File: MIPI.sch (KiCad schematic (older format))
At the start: 42 parts, among them J8 49F-1201GYD2NL, J9 MIPI, U1 AllWinner-S3(FBGA-234), Y2 32.768kHz, Y3 24MHz

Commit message: no drc error
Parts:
- R78, R79, R80, R81, R82, R83, R84, R86, R87, R88, R89, R90, R91, R92, R93, R94: footprint otter:C_0402 -> otter:R_0402
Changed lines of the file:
@@
 F 0 "R81" V 2150 1750 50  0000 C CNN
 F 1 "22" V 2150 2050 50  0000 C CNN
-F 2 "otter:C_0402" H 2200 1900 50  0001 C CNN
+F 2 "otter:R_0402" H 2200 1900 50  0001 C CNN
 F 3 "~" H 2200 1900 50  0001 C CNN
 	1    2200 1900
@@
 F 0 "R78" H 1092 3696 50  0000 R CNN
 F 1 "200k" H 1092 3605 50  0000 R CNN
-F 2 "otter:C_0402" H 1150 3650 50  0001 C CNN
+F 2 "otter:R_0402" H 1150 3650 50  0001 C CNN
 F 3 "~" H 1150 3650 50  0001 C CNN
 	1    1150 3650
@@
 F 0 "R87" V 7700 1300 50  0000 C CNN
 F 1 "2k2" V 7700 1650 50  0000 C CNN
-F 2 "otter:C_0402" H 7750 1450 50  0001 C CNN
+F 2 "otter:R_0402" H 7750 1450 50  0001 C CNN
 F 3 "~" H 7750 1450 50  0001 C CNN
 	1    7750 1450
@@
 F 0 "R88" V 7400 1300 50  0000 C CNN
 F 1 "2k2" V 7400 1650 50  0000 C CNN
-F 2 "otter:C_0402" H 7450 1450 50  0001 C CNN
+F 2 "otter:R_0402" H 7450 1450 50  0001 C CNN
 F 3 "~" H 7450 1450 50  0001 C CNN
 	1    7450 1450
@@
 F 0 "R89" V 4750 4050 50  0000 C CNN
 F 1 "6k04" V 4750 4400 50  0000 C CNN
-F 2 "otter:C_0402" H 4800 4200 50  0001 C CNN
+F 2 "otter:R_0402" H 4800 4200 50  0001 C CNN
 F 3 "~" H 4800 4200 50  0001 C CNN
 	1    4800 4200
@@
 F 0 "R79" V 1800 4600 50  0000 C CNN
 F 1 "2k2" V 1800 4900 50  0000 C CNN
-F 2 "otter:C_0402" H 1850 4750 50  0001 C CNN
+F 2 "otter:R_0402" H 1850 4750 50  0001 C CNN
 F 3 "~" H 1850 4750 50  0001 C CNN
 	1    1850 4750
@@
 F 0 "R82" H 2350 5550 50  0000 L CNN
 F 1 "240" H 2300 5450 50  0000 L CNN
-F 2 "otter:C_0402" H 2500 5500 50  0001 C CNN
+F 2 "otter:R_0402" H 2500 5500 50  0001 C CNN
 F 3 "~" H 2500 5500 50  0001 C CNN
 	1    2500 5500
@@
 F 0 "R83" H 2659 5546 50  0000 L CNN
 F 1 "240" H 2659 5455 50  0000 L CNN
-F 2 "otter:C_0402" H 2600 5500 50  0001 C CNN
+F 2 "otter:R_0402" H 2600 5500 50  0001 C CNN
 F 3 "~" H 2600 5500 50  0001 C CNN
 	1    2600 5500
@@
 F 0 "R84" H 4141 4654 50  0000 R CNN
 F 1 "10M" H 4141 4745 50  0000 R CNN
-F 2 "otter:C_0402" H 4200 4700 50  0001 C CNN
+F 2 "otter:R_0402" H 4200 4700 50  0001 C CNN
 F 3 "~" H 4200 4700 50  0001 C CNN
 	1    4200 4700
@@
 F 0 "R86" V 4400 4700 50  0000 C CNN
 F 1 "5k1" V 4400 4450 50  0000 C CNN
-F 2 "otter:C_0402" H 4400 4450 50  0001 C CNN
+F 2 "otter:R_0402" H 4400 4450 50  0001 C CNN
 F 3 "~" H 4400 4450 50  0001 C CNN
 	1    4400 4450
@@
 F 0 "R91" V 9150 2700 50  0000 C CNN
 F 1 "51" V 9100 2450 50  0000 C CNN
-F 2 "otter:C_0402" H 9100 2450 50  0001 C CNN
+F 2 "otter:R_0402" H 9100 2450 50  0001 C CNN
 F 3 "~" H 9100 2450 50  0001 C CNN
 	1    9100 2450
@@
 F 0 "R90" V 9050 2800 50  0000 C CNN
 F 1 "51" V 9100 2550 50  0000 C CNN
-F 2 "otter:C_0402" H 9100 2550 50  0001 C CNN
+F 2 "otter:R_0402" H 9100 2550 50  0001 C CNN
 F 3 "~" H 9100 2550 50  0001 C CNN
 	1    9100 2550
@@
 F 0 "R93" V 9150 2300 50  0000 C CNN
 F 1 "51" V 9100 2050 50  0000 C CNN
-F 2 "otter:C_0402" H 9100 2050 50  0001 C CNN
+F 2 "otter:R_0402" H 9100 2050 50  0001 C CNN
 F 3 "~" H 9100 2050 50  0001 C CNN
 	1    9100 2050
@@
 F 0 "R92" V 9050 2400 50  0000 C CNN
 F 1 "51" V 9100 2150 50  0000 C CNN
-F 2 "otter:C_0402" H 9100 2150 50  0001 C CNN
+F 2 "otter:R_0402" H 9100 2150 50  0001 C CNN
 F 3 "~" H 9100 2150 50  0001 C CNN
 	1    9100 2150
@@
 F 0 "R80" V 1800 4950 50  0000 C CNN
 F 1 "2k2" V 1800 5250 50  0000 C CNN
-F 2 "otter:C_0402" H 1850 5100 50  0001 C CNN
+F 2 "otter:R_0402" H 1850 5100 50  0001 C CNN
 F 3 "~" H 1850 5100 50  0001 C CNN
 	1    1850 5100
@@
 F 0 "R94" V 9900 4300 50  0000 C CNN
 F 1 "51" V 10100 4300 50  0000 C CNN
-F 2 "otter:C_0402" H 10000 4300 50  0001 C CNN
+F 2 "otter:R_0402" H 10000 4300 50  0001 C CNN
 F 3 "~" H 10000 4300 50  0001 C CNN
 	1    10000 4300

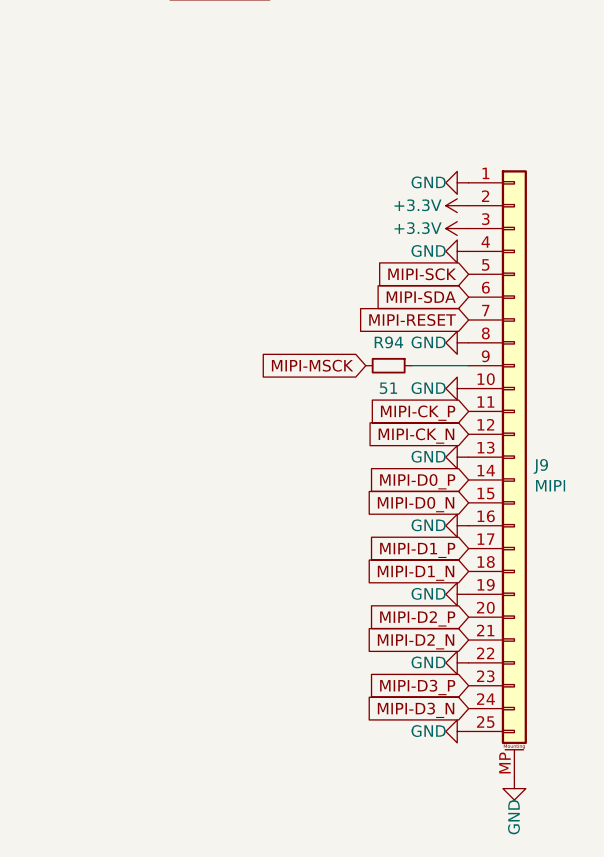
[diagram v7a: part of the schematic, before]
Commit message: fixed axp bug, fixed schematics, fixed eeprom
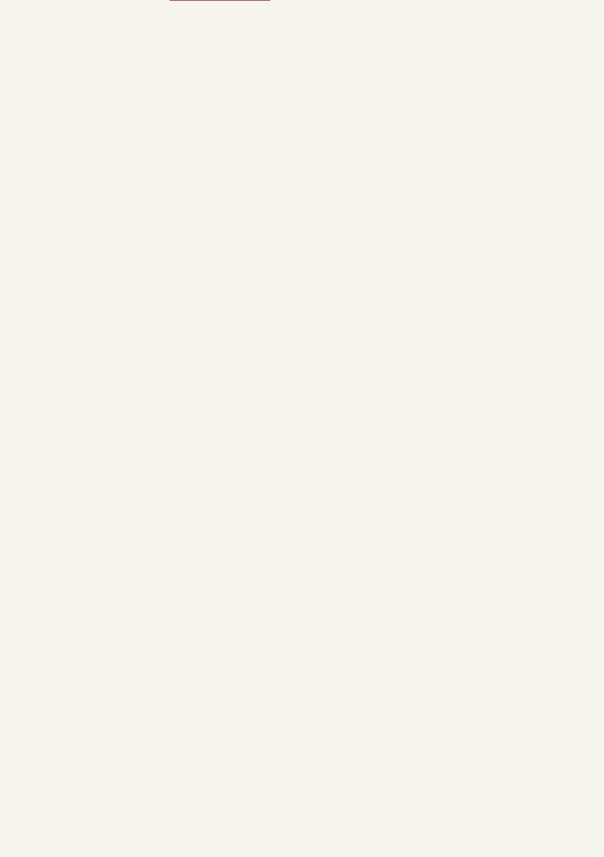
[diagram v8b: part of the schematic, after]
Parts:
- removed J9: MIPI, otter:FH35C-25S, symbol Connector_Generic_MountingPin:Conn_01x25_MountingPin
- removed R94: 51, otter:R_0402, symbol Device:R_Small
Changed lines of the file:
@@
-$EndComp
-$Comp
-L S3-OLinuXino_Rev_A:GND #PWR?
-U 1 1 621FAC24
-P 10350 3800
-AR Path="/5D8A1FAC/621FAC24" Ref="#PWR?"  Part="1"
-AR Path="/621FAC24" Ref="#PWR?"  Part="1"
-AR Path="/620E795B/621FAC24" Ref="#PWR0260"  Part="1"
-F 0 "#PWR0260" H 10350 3550 50  0001 C CNN
-F 1 "GND" V 10350 3625 50  0000 C CNN
-F 2 "" H 10350 3800 60  0000 C CNN
-F 3 "" H 10350 3800 60  0000 C CNN
-	1    10350 3800
-	0    1    1    0
-$EndComp
-$Comp
-L S3-OLinuXino_Rev_A:GND #PWR?
-U 1 1 621FAC2A
-P 10350 3500
-AR Path="/5D8A1FAC/621FAC2A" Ref="#PWR?"  Part="1"
-AR Path="/621FAC2A" Ref="#PWR?"  Part="1"
-AR Path="/620E795B/621FAC2A" Ref="#PWR0261"  Part="1"
-F 0 "#PWR0261" H 10350 3250 50  0001 C CNN
-F 1 "GND" V 10350 3325 50  0000 C CNN
-F 2 "" H 10350 3500 60  0000 C CNN
-F 3 "" H 10350 3500 60  0000 C CNN
-	1    10350 3500
-	0    1    1    0
-$EndComp
-$Comp
-L S3-OLinuXino_Rev_A:GND #PWR?
-U 1 1 621FAC30
-P 10350 4200
-AR Path="/5D8A1FAC/621FAC30" Ref="#PWR?"  Part="1"
-AR Path="/621FAC30" Ref="#PWR?"  Part="1"
-AR Path="/620E795B/621FAC30" Ref="#PWR0262"  Part="1"
-F 0 "#PWR0262" H 10350 3950 50  0001 C CNN
-F 1 "GND" V 10350 4025 50  0000 C CNN
-F 2 "" H 10350 4200 60  0000 C CNN
-F 3 "" H 10350 4200 60  0000 C CNN
-	1    10350 4200
-	0    1    1    0
 $EndComp
 $Comp
@@
 	0    1    -1   0
 $EndComp
-Text GLabel 10350 4000 0    50   Input ~ 0
-MIPI-SDA
-Text GLabel 10350 3900 0    50   Input ~ 0
-MIPI-SCK
 $Comp
 L otter:AllWinner-S3(FBGA-234) U?
@@
 Text GLabel 4100 2300 2    50   Input ~ 0
 MIPI-D3_N
-Text GLabel 10350 4500 0    50   Input ~ 0
-MIPI-CK_P
-Text GLabel 10350 4600 0    50   Input ~ 0
-MIPI-CK_N
-Text GLabel 10350 4800 0    50   Input ~ 0
-MIPI-D0_P
-Text GLabel 10350 4900 0    50   Input ~ 0
-MIPI-D0_N
-Text GLabel 10350 5100 0    50   Input ~ 0
-MIPI-D1_P
-Text GLabel 10350 5200 0    50   Input ~ 0
-MIPI-D1_N
-Text GLabel 10350 5400 0    50   Input ~ 0
-MIPI-D2_P
-Text GLabel 10350 5500 0    50   Input ~ 0
-MIPI-D2_N
-Text GLabel 10350 5700 0    50   Input ~ 0
-MIPI-D3_P
-Text GLabel 10350 5800 0    50   Input ~ 0
-MIPI-D3_N
-Text GLabel 10350 4100 0    50   Input ~ 0
-MIPI-RESET
 Text GLabel 4100 3600 2    50   Input ~ 0
 EPHY_TX_P
@@
 Wire Wire Line
 	4100 3400 5300 3400
-Text GLabel 9900 4300 0    50   Input ~ 0
-MIPI-MSCK
-$Comp
-L Connector_Generic_MountingPin:Conn_01x25_MountingPin J9
-U 1 1 60E65401
-P 10550 4700
-F 0 "J9" H 10638 4664 50  0000 L CNN
-F 1 "MIPI" H 10638 4573 50  0000 L CNN
-F 2 "otter:FH35C-25S" H 10550 4700 50  0001 C CNN
-F 3 "~" H 10550 4700 50  0001 C CNN
-	1    10550 4700
-	1    0    0    -1
-$EndComp
-$Comp
-L S3-OLinuXino_Rev_A:GND #PWR?
-U 1 1 60E67C55
-P 10350 4400
-AR Path="/5D8A1FAC/60E67C55" Ref="#PWR?"  Part="1"
-AR Path="/60E67C55" Ref="#PWR?"  Part="1"
-AR Path="/620E795B/60E67C55" Ref="#PWR0263"  Part="1"
-F 0 "#PWR0263" H 10350 4150 50  0001 C CNN
-F 1 "GND" V 10350 4225 50  0000 C CNN
-F 2 "" H 10350 4400 60  0000 C CNN
-F 3 "" H 10350 4400 60  0000 C CNN
-	1    10350 4400
-	0    1    1    0
-$EndComp
-$Comp
-L S3-OLinuXino_Rev_A:GND #PWR?
-U 1 1 60E72A38
-P 10350 4700
-AR Path="/5D8A1FAC/60E72A38" Ref="#PWR?"  Part="1"
-AR Path="/60E72A38" Ref="#PWR?"  Part="1"
-AR Path="/620E795B/60E72A38" Ref="#PWR0264"  Part="1"
-F 0 "#PWR0264" H 10350 4450 50  0001 C CNN
-F 1 "GND" V 10350 4525 50  0000 C CNN
-F 2 "" H 10350 4700 60  0000 C CNN
-F 3 "" H 10350 4700 60  0000 C CNN
-	1    10350 4700
-	0    1    1    0
-$EndComp
-$Comp
-L S3-OLinuXino_Rev_A:GND #PWR?
-U 1 1 60E781AE
-P 10350 5000
-AR Path="/5D8A1FAC/60E781AE" Ref="#PWR?"  Part="1"
-AR Path="/60E781AE" Ref="#PWR?"  Part="1"
-AR Path="/620E795B/60E781AE" Ref="#PWR0288"  Part="1"
-F 0 "#PWR0288" H 10350 4750 50  0001 C CNN
-F 1 "GND" V 10350 4825 50  0000 C CNN
-F 2 "" H 10350 5000 60  0000 C CNN
-F 3 "" H 10350 5000 60  0000 C CNN
-	1    10350 5000
-	0    1    1    0
-$EndComp
-$Comp
-L S3-OLinuXino_Rev_A:GND #PWR?
-U 1 1 60E7D9BE
-P 10350 5300
-AR Path="/5D8A1FAC/60E7D9BE" Ref="#PWR?"  Part="1"
-AR Path="/60E7D9BE" Ref="#PWR?"  Part="1"
-AR Path="/620E795B/60E7D9BE" Ref="#PWR0289"  Part="1"
-F 0 "#PWR0289" H 10350 5050 50  0001 C CNN
-F 1 "GND" V 10350 5125 50  0000 C CNN
-F 2 "" H 10350 5300 60  0000 C CNN
-F 3 "" H 10350 5300 60  0000 C CNN
-	1    10350 5300
-	0    1    1    0
-$EndComp
-$Comp
-L S3-OLinuXino_Rev_A:GND #PWR?
-U 1 1 60E832C7
-P 10350 5600
-AR Path="/5D8A1FAC/60E832C7" Ref="#PWR?"  Part="1"
-AR Path="/60E832C7" Ref="#PWR?"  Part="1"
-AR Path="/620E795B/60E832C7" Ref="#PWR0290"  Part="1"
-F 0 "#PWR0290" H 10350 5350 50  0001 C CNN
-F 1 "GND" V 10350 5425 50  0000 C CNN
-F 2 "" H 10350 5600 60  0000 C CNN
-F 3 "" H 10350 5600 60  0000 C CNN
-	1    10350 5600
-	0    1    1    0
-$EndComp
-$Comp
-L S3-OLinuXino_Rev_A:GND #PWR?
-U 1 1 60E88B22
-P 10350 5900
-AR Path="/5D8A1FAC/60E88B22" Ref="#PWR?"  Part="1"
-AR Path="/60E88B22" Ref="#PWR?"  Part="1"
-AR Path="/620E795B/60E88B22" Ref="#PWR0291"  Part="1"
-F 0 "#PWR0291" H 10350 5650 50  0001 C CNN
-F 1 "GND" V 10350 5725 50  0000 C CNN
-F 2 "" H 10350 5900 60  0000 C CNN
-F 3 "" H 10350 5900 60  0000 C CNN
-	1    10350 5900
-	0    1    1    0
-$EndComp
-$Comp
-L S3-OLinuXino_Rev_A:GND #PWR?
-U 1 1 60E8E32D
-P 10550 6100
-AR Path="/5D8A1FAC/60E8E32D" Ref="#PWR?"  Part="1"
-AR Path="/60E8E32D" Ref="#PWR?"  Part="1"
-AR Path="/620E795B/60E8E32D" Ref="#PWR0292"  Part="1"
-F 0 "#PWR0292" H 10550 5850 50  0001 C CNN
-F 1 "GND" V 10550 5925 50  0000 C CNN
-F 2 "" H 10550 6100 60  0000 C CNN
-F 3 "" H 10550 6100 60  0000 C CNN
-	1    10550 6100
-	1    0    0    -1
-$EndComp
-$Comp
-L S3-OLinuXino_Rev_A:+3.3V #PWR?
-U 1 1 60E9A477
-P 10350 3600
-AR Path="/5D8A1FAC/60E9A477" Ref="#PWR?"  Part="1"
-AR Path="/60E9A477" Ref="#PWR?"  Part="1"
-AR Path="/620E795B/60E9A477" Ref="#PWR0293"  Part="1"
-F 0 "#PWR0293" H 10350 3450 50  0001 C CNN
-F 1 "+3.3V" V 10350 3825 50  0000 C CNN
-F 2 "" H 10350 3600 60  0000 C CNN
-F 3 "" H 10350 3600 60  0000 C CNN
-	1    10350 3600
-	0    -1   1    0
-$EndComp
-$Comp
-L S3-OLinuXino_Rev_A:+3.3V #PWR?
-U 1 1 60E9FB5F
-P 10350 3700
-AR Path="/5D8A1FAC/60E9FB5F" Ref="#PWR?"  Part="1"
-AR Path="/60E9FB5F" Ref="#PWR?"  Part="1"
-AR Path="/620E795B/60E9FB5F" Ref="#PWR0294"  Part="1"
-F 0 "#PWR0294" H 10350 3550 50  0001 C CNN
-F 1 "+3.3V" V 10350 3925 50  0000 C CNN
-F 2 "" H 10350 3700 60  0000 C CNN
-F 3 "" H 10350 3700 60  0000 C CNN
-	1    10350 3700
-	0    -1   1    0
-$EndComp
-$Comp
-L Device:R_Small R?
-U 1 1 60ECC72B
-P 10000 4300
-AR Path="/60ECC72B" Ref="R?"  Part="1"
-AR Path="/620E795B/60ECC72B" Ref="R94"  Part="1"
-F 0 "R94" V 9900 4300 50  0000 C CNN
-F 1 "51" V 10100 4300 50  0000 C CNN
-F 2 "otter:R_0402" H 10000 4300 50  0001 C CNN
-F 3 "~" H 10000 4300 50  0001 C CNN
-	1    10000 4300
-	0    1    1    0
-$EndComp
-Wire Wire Line
-	10100 4300 10350 4300
 Wire Wire Line
 	4100 5300 4400 5300
